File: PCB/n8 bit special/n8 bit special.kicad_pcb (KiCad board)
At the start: 2 copper layers, 99.7 x 97.8 mm, 36 parts, among them J1 PowerPort, J2 PORT0, J3 PORT2, J4 PORT1, J5 PORT3, J6 Conn_02x08_Odd_Even, SW1 SW_Push_Dual, U1 W65C02SxP, U2 CY62256-70PC, U3 CY62256-70PC, U4 28C256, U5 74LS21, U6 22V10C, U7 DS1813, X1 2Mhz

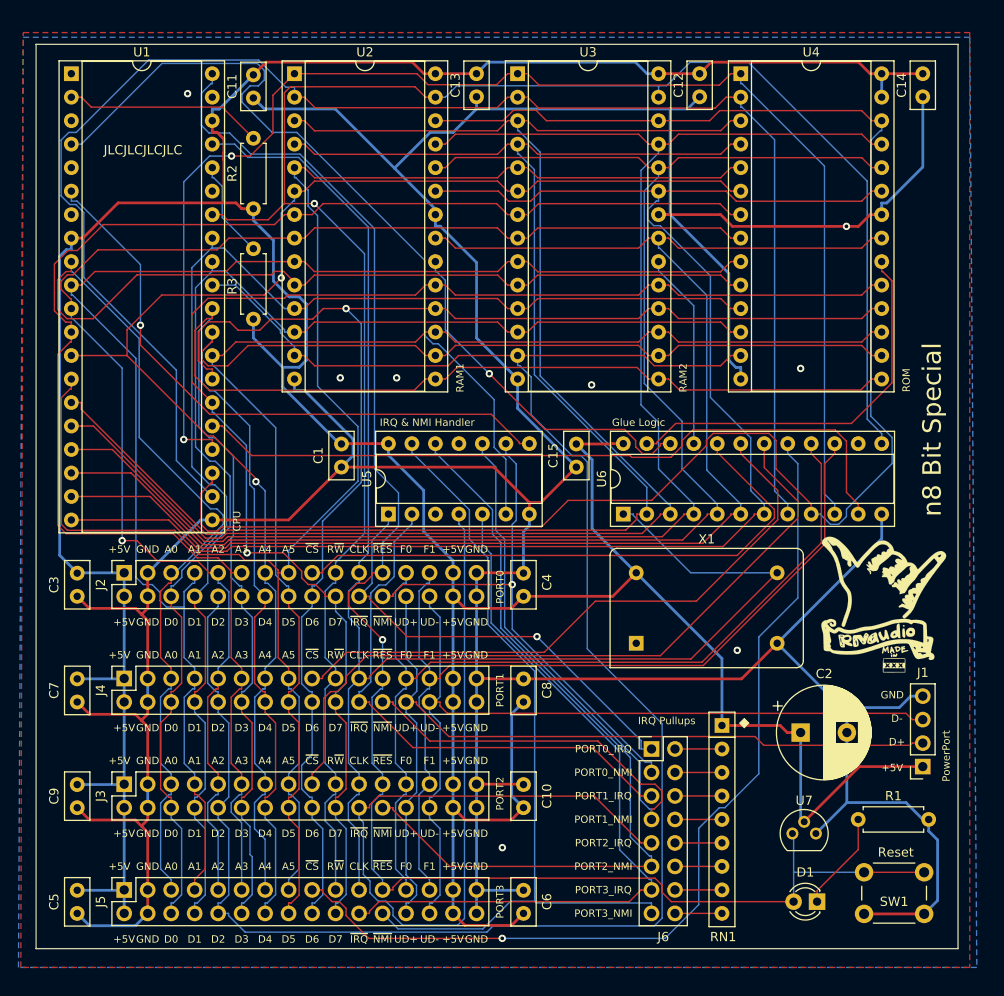
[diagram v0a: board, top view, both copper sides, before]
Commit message: version 2 of the PCB
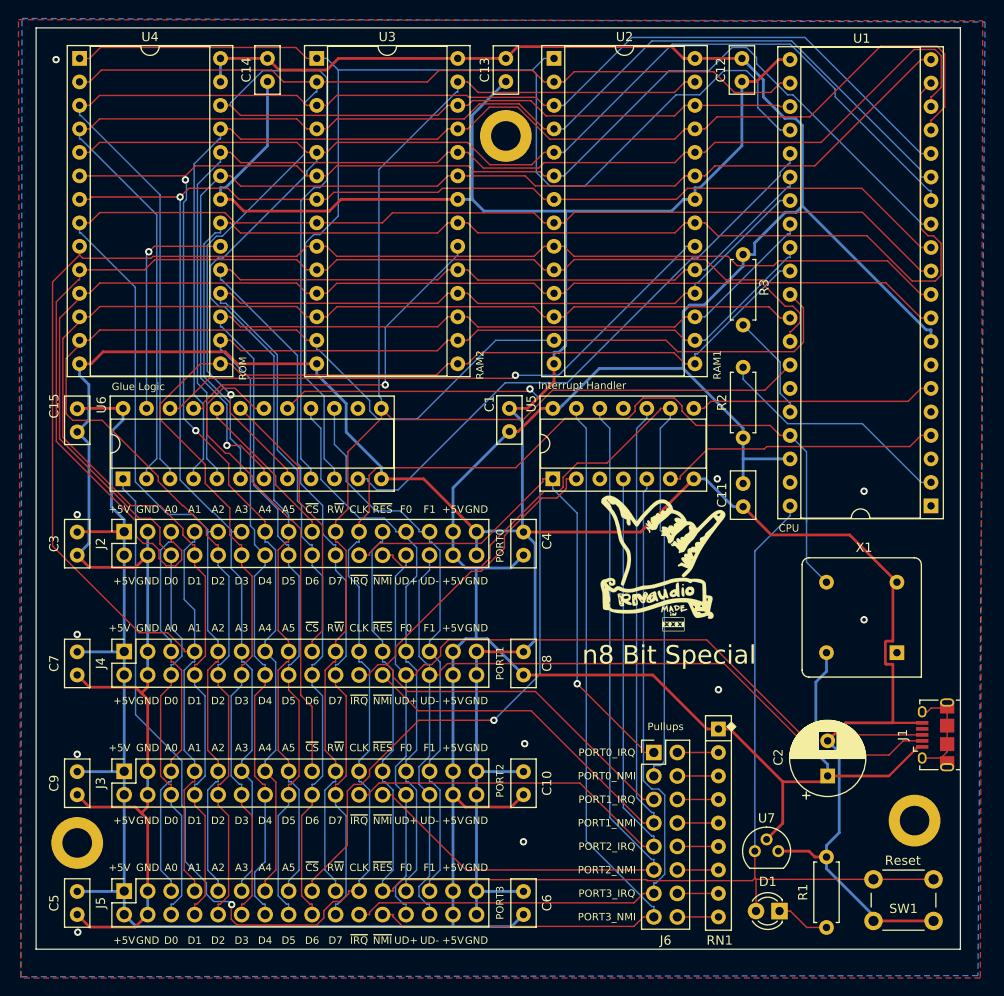
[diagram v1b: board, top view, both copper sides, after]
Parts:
- added REF1: MountingHole_3.2mm_M3_DIN965_Pad, MountingHole:MountingHole_3.2mm_M3_DIN965_Pad, F.Cu at (91.4, 128.3)
- added REF2: MountingHole_3.2mm_M3_DIN965_Pad, MountingHole:MountingHole_3.2mm_M3_DIN965_Pad, F.Cu at (137.8, 51.8)
- added REF3: MountingHole_3.2mm_M3_DIN965_Pad, MountingHole:MountingHole_3.2mm_M3_DIN965_Pad, F.Cu at (182.0, 125.9)
- C2: value 1000uF -> 470uF; footprint Capacitor_THT:CP_Radial_D10.0mm_P5.00mm -> Capacitor_THT:CP_Radial_D8.0mm_P3.80mm
- J1: value PowerPort -> USB_B_Micro; footprint Connector_PinSocket_2.54mm:PinSocket_1x04_P2.54mm_Vertical -> Connector_USB:USB_Micro-B_Amphenol_10118194_Horizontal
- X1: value 2Mhz -> 4Mhz; footprint Oscillator:Oscillator_DIP-14 -> Oscillator:Oscillator_DIP-8
- moved U1 104.1 mm to (183.8, 91.8), turned to 180 degrees
- moved U4 71.5 mm to (91.7, 43.4)
- moved C14 70.9 mm to (112.0, 43.4)
- moved C11 69.0 mm to (163.4, 89.4)
- moved R2 58.5 mm to (163.4, 76.8)
- moved U6 54.2 mm to (96.4, 88.9)
- moved C15 54.1 mm to (91.4, 83.8)
- moved R3 53.6 mm to (163.4, 72.3), turned to 90 degrees
- moved X1 28.2 mm to (180.1, 107.7), turned to 90 degrees
- moved U2 28.1 mm to (143.0, 43.4)
- moved G*** 24.3 mm to (154.7, 97.4)
- moved U3 21.8 mm to (117.3, 43.4)
- moved C1 19.2 mm to (138.2, 81.3), turned to 270 degrees
- moved U5 18.2 mm to (142.9, 88.9)
- moved R1 12.2 mm to (172.5, 137.4), turned to 90 degrees
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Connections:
- J1 pad 2: USB_D+ -> USB_D-
- J1 pad 3: USB_D- -> USB_D+
- J1 pad 4: GND -> Net-(J1-Pad4)
- X1 pad 8: CLK -> +5V
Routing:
- net /A13: track 184.3 -> 122.8 mm
- net ~IRQ: track 88.0 -> 30.3 mm
- net /D2: track 218.0 -> 169.2 mm
- net /A11: track 169.3 -> 121.2 mm, vias 0 -> 1
- net ~PORT0_CS: track 63.3 -> 17.7 mm
- net /A12: track 174.3 -> 132.7 mm, vias 0 -> 1
- net ~NMI: track 66.7 -> 26.5 mm, vias 1 -> 0
- net FUTURE0: track 99.9 -> 62.0 mm
- net /A1: track 154.4 -> 192.2 mm
- net /A9: track 166.0 -> 128.4 mm
- net ~PORT1_CS: track 67.5 -> 30.4 mm
- net /A4: track 155.6 -> 192.2 mm
- net FUTURE1: track 97.7 -> 61.8 mm
- net R~W: track 205.8 -> 170.3 mm, vias 1 -> 0
- net /A8: track 166.0 -> 135.0 mm
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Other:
- board size 99.7 x 97.8 mm -> 99.9 x 99.6 mm
- board text added: "Interrupt Handler"
- board text added: "Pullups"
- board text added: "by Nate Rivard https://github.com/nrivard/lmaos Version 2 Mar 2021"
- board text removed: "D+"
- board text removed: "D-"
- board text removed: "IRQ & NMI Handler"
- board text removed: "IRQ Pullups"
- board text removed: "JLCJLCJLCJLC"
- board text removed: "PowerPort"
- board text removed: "by Nate Rivard https://github.com/nrivard/lmaos Version 1 Mar 2021"
